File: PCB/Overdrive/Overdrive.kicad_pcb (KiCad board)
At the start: 2 copper layers, 89 x 76.3 mm, 47 parts, among them J1 Alimentación, J2 Entrada, J3 Salida, J4 LM1117_3.3V, SW2 BT_sw, U1 TL072, U2 TL072

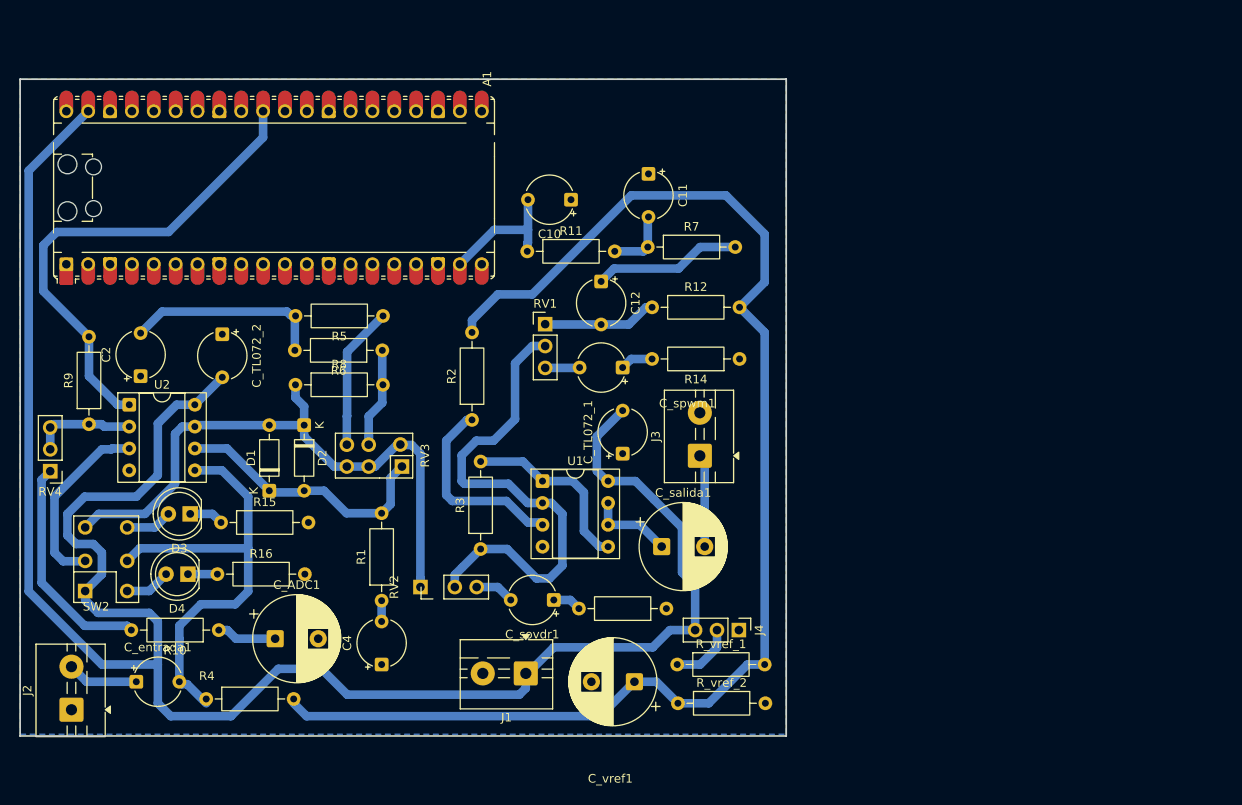
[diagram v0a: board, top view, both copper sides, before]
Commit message: A
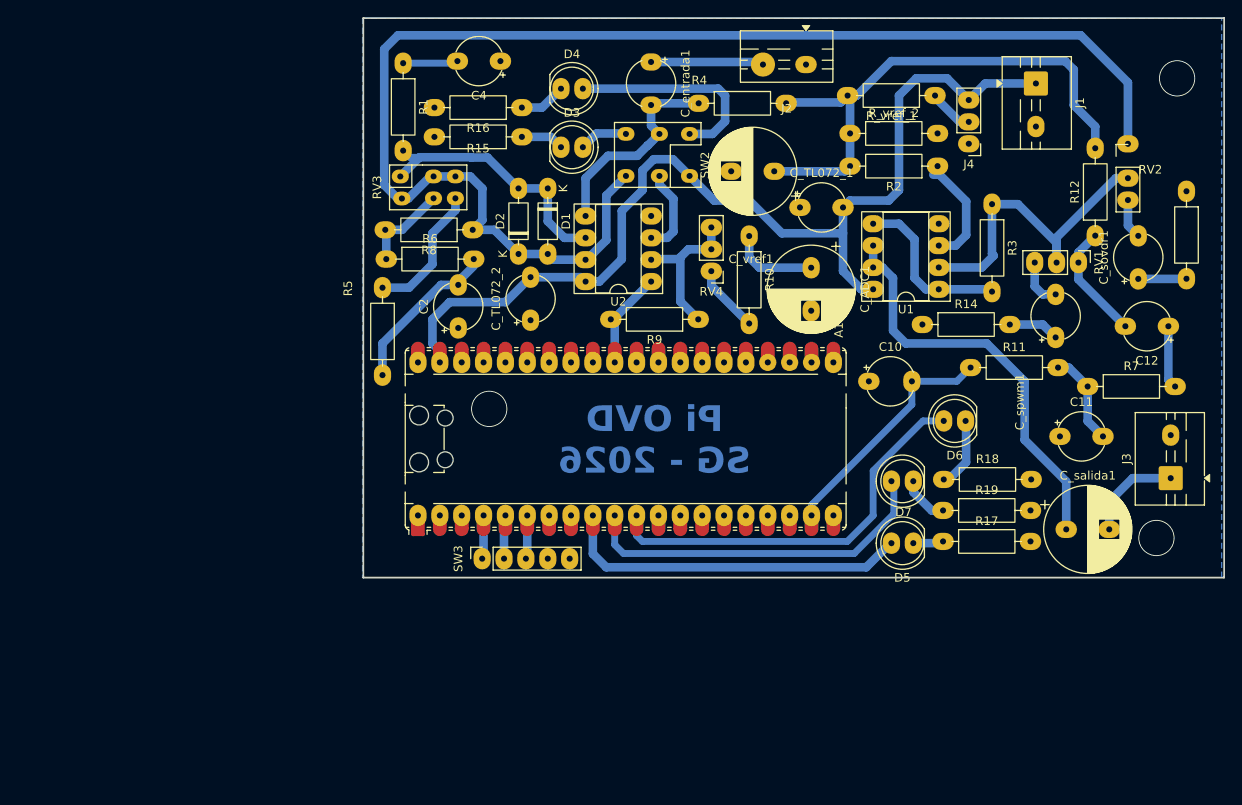
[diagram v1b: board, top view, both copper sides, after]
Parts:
- added D5: LED, LED_THT:LED_D5.0mm_FlatTop, F.Cu at (134.3, 175.4)
- added D6: LED, LED_THT:LED_D5.0mm_FlatTop, F.Cu at (140.3, 161.2)
- added D7: LED, LED_THT:LED_D5.0mm_FlatTop, F.Cu at (134.3, 168.2)
- added R17: R_US, Resistor_THT:R_Axial_DIN0207_L6.3mm_D2.5mm_P10.16mm_Horizontal, F.Cu at (137.7, 175.2)
- added R18: R_US, Resistor_THT:R_Axial_DIN0207_L6.3mm_D2.5mm_P10.16mm_Horizontal, F.Cu at (137.8, 168.0)
- added R19: R_US, Resistor_THT:R_Axial_DIN0207_L6.3mm_D2.5mm_P10.16mm_Horizontal, F.Cu at (137.7, 171.6)
- added SW3: RotaryEncoder_Switch, Connector_PinSocket_2.54mm:PinSocket_1x05_P2.54mm_Vertical, F.Cu at (84.2, 177.2)
- moved J2 113.6 mm to (121.8, 119.8), turned to 180 degrees
- moved RV2 95.0 mm to (159.2, 130.5), turned to 0 degrees
- moved C_entrada1 93.6 mm to (103.8, 119.5), turned to -90 degrees
- moved J1 90.6 mm to (148.5, 122.0), turned to -90 degrees
- moved R4 89.8 mm to (109.3, 124.3)
- moved SW2 83.3 mm to (107.3, 130.4), turned to -90 degrees
- moved RV4 80.2 mm to (110.8, 143.8)
- moved C_sovdr1 77.5 mm to (160.4, 144.7), turned to 90 degrees
- moved R13 77.5 mm to (166.0, 134.5), turned to -90 degrees
- moved R10 76.8 mm to (115.2, 139.7), turned to -90 degrees
- moved C_ADC1 75.7 mm to (122.4, 143.4), turned to -90 degrees
- moved R_vref_1 72.6 mm to (136.8, 123.4), turned to 180 degrees
- moved R9 71.8 mm to (109.3, 149.4), turned to 180 degrees
- moved R3 71.7 mm to (143.4, 136.0), turned to -90 degrees
- moved C4 71.4 mm to (86.3, 119.4), turned to 180 degrees
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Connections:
- A1 pad 10: unconnected-(A1-GPIO7-Pad10) -> Net-(A1-GPIO7)
- A1 pad 11: unconnected-(A1-GPIO8-Pad11) -> Net-(A1-GPIO8)
- A1 pad 4: unconnected-(A1-GPIO2-Pad4) -> Net-(A1-GPIO2)
- A1 pad 5: unconnected-(A1-GPIO3-Pad5) -> Net-(A1-GPIO3)
- A1 pad 6: unconnected-(A1-GPIO4-Pad6) -> Net-(A1-GPIO4)
- A1 pad 9: unconnected-(A1-GPIO6-Pad9) -> Net-(A1-GPIO6)
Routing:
- net Vcc: track 241.9 -> 118.0 mm
- net Vref: track 155.6 -> 63.4 mm
- net Net-(D1-A): track 72.1 -> 157.5 mm
- net Net-(A1-GPIO8): track 0.00 -> 47.1 mm
- net ADC_IN: track 57.2 -> 11.7 mm
- net Net-(A1-GPIO7): track 0.00 -> 42.1 mm
- net Net-(A1-GPIO6): track 0.00 -> 41.0 mm
- net Net-(U1B--): track 9.81 -> 48.4 mm
- net Net-(SW2A-A): track 53.4 -> 24.5 mm
- net Net-(U1A--): track 58.2 -> 38.7 mm
- net Net-(D4-A): track 5.33 -> 24.6 mm
- net Net-(R10-Pad2): track 26.1 -> 7.90 mm
- net PWM_out: track 15.6 -> 27.9 mm
- net Net-(SW2A-B): track 21.5 -> 10.0 mm
- net Net-(U1A-+): track 22.9 -> 12.7 mm
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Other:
- board size 89 x 76.3 mm -> 100 x 65 mm
- board text added: "Pi OVD SG - 2026"

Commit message: A
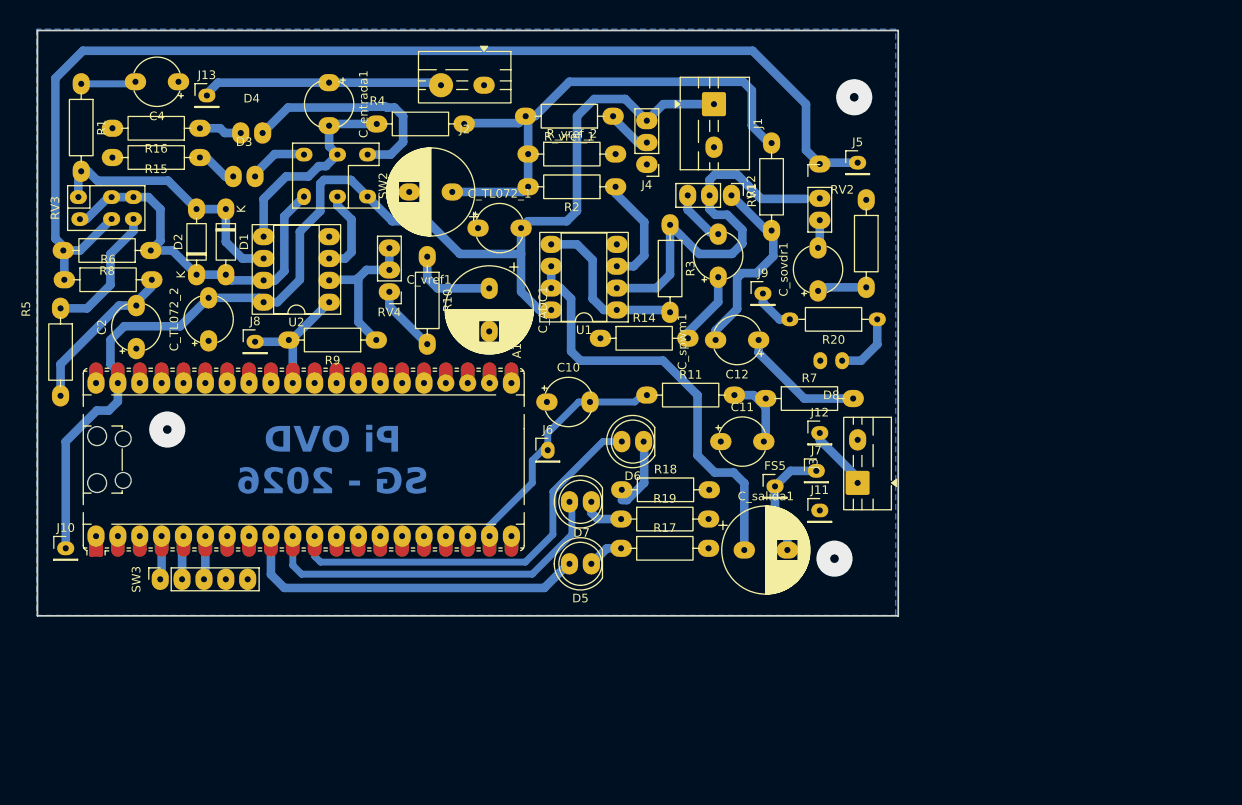
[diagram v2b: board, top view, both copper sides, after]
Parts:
- added D8: LED, LED_THT:LED_D5.0mm_FlatTop, F.Cu at (126.0, 154.2)
- added FS5: OUT, Connector_PinHeader_2.54mm:PinHeader_1x01_P2.54mm_Vertical, F.Cu at (118.2, 168.8)
- added J10: FS2, Connector_PinHeader_2.54mm:PinHeader_1x01_P2.54mm_Vertical, F.Cu at (35.8, 176.0)
- added J11: FS3, Connector_PinHeader_2.54mm:PinHeader_1x01_P2.54mm_Vertical, F.Cu at (123.4, 171.6)
- added J12: FS6, Connector_PinHeader_2.54mm:PinHeader_1x01_P2.54mm_Vertical, F.Cu at (123.4, 162.6)
- added J13: FS4, Connector_PinHeader_2.54mm:PinHeader_1x01_P2.54mm_Vertical, F.Cu at (52.2, 123.4)
- added J5: OVD, Connector_PinHeader_2.54mm:PinHeader_1x01_P2.54mm_Vertical, F.Cu at (127.8, 131.2)
- added J6: PWM, Connector_PinHeader_2.54mm:PinHeader_1x01_P2.54mm_Vertical, F.Cu at (91.8, 164.6)
- added J7: OUT, Connector_PinHeader_2.54mm:PinHeader_1x01_P2.54mm_Vertical, F.Cu at (123.0, 167.0)
- added J8: ADC_in, Connector_PinHeader_2.54mm:PinHeader_1x01_P2.54mm_Vertical, F.Cu at (57.8, 152.0)
- added J9: FS1, Connector_PinHeader_2.54mm:PinHeader_1x01_P2.54mm_Vertical, F.Cu at (116.8, 146.4)
- added R20: R_US, Resistor_THT:R_Axial_DIN0207_L6.3mm_D2.5mm_P10.16mm_Horizontal, F.Cu at (130.1, 149.4)
- moved C12 47.6 mm to (116.3, 151.8)
- moved RV1 41.1 mm to (113.1, 135.0)
- moved C_spwm1 39.8 mm to (111.6, 144.5)
- moved C11 39.4 mm to (111.9, 163.6)
- moved D3 38.2 mm to (55.3, 132.8)
- moved R11 37.7 mm to (103.3, 158.2)
- moved R12 37.6 mm to (117.8, 139.1)
- moved D4 37.6 mm to (56.1, 127.8)
- moved C2 37.5 mm to (44.0, 152.8)
- moved C_ADC1 37.5 mm to (85.0, 145.8)
- moved C_vref1 37.5 mm to (80.7, 134.6)
- moved D2 37.5 mm to (51.0, 144.2)
- moved D6 37.5 mm to (102.9, 163.6)
- moved J4 37.5 mm to (103.3, 131.4)
- moved R10 37.5 mm to (77.8, 142.1)
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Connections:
- net Net-(J2-Pin_2) renamed /In
- C_salida1 pad 2: Net-(J3-Pin_1) -> /Out_p
- J3 pad 1: Net-(J3-Pin_1) -> Net-(J12-Pin_1)
- R6 pad 1: Net-(R6-Pad1) -> Net-(J5-Pin_1)
- R8 pad 2: Net-(R6-Pad1) -> Net-(J5-Pin_1)
- RV2 pad 1: Net-(D1-A) -> Net-(J5-Pin_1)
- RV3 pad 5: Net-(R6-Pad1) -> Net-(J5-Pin_1)
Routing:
- net Net-(J5-Pin_1): track 0.00 -> 134.3 mm
- net Net-(D1-A): track 157.5 -> 43.3 mm
- net Vcc: track 118.0 -> 141.1 mm
- net /In: track 13.1 -> 28.1 mm
- net /Out_p: track 0.00 -> 13.5 mm
- net Net-(J3-Pin_1): track 11.5 -> 0.00 mm
- net Net-(R6-Pad1): track 10.7 -> 0.00 mm
- net Net-(C12-Pad2): track 13.6 -> 22.6 mm
- net Net-(J12-Pin_1): track 0.00 -> 8.02 mm
- net Net-(D8-K): track 0.00 -> 7.78 mm
- net Net-(C12-Pad1): track 7.32 -> 14.7 mm
- net Net-(U1A--): track 38.7 -> 45.9 mm
- net Net-(J9-Pin_1): track 0.00 -> 5.00 mm
- net ADC_IN: track 11.7 -> 15.7 mm
- net Net-(C_spwm1-Pad1): track 5.94 -> 8.76 mm
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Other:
- board size 100 x 65 mm -> 100 x 68 mm
